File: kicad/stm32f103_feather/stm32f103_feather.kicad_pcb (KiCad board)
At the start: 2 copper layers, 50.8 x 22.9 mm, 34 parts, among them J1 Bottom-conn, J2 Top-conn, J3 Debug-conn, J4 USB_B_Micro, J5 JST-LiPo-conn, SW1 SW_Push, U1 STM32F103CBTx, U2 AMS1117-3.3, U3 MCP73831-2-OT, Y1 8MHz

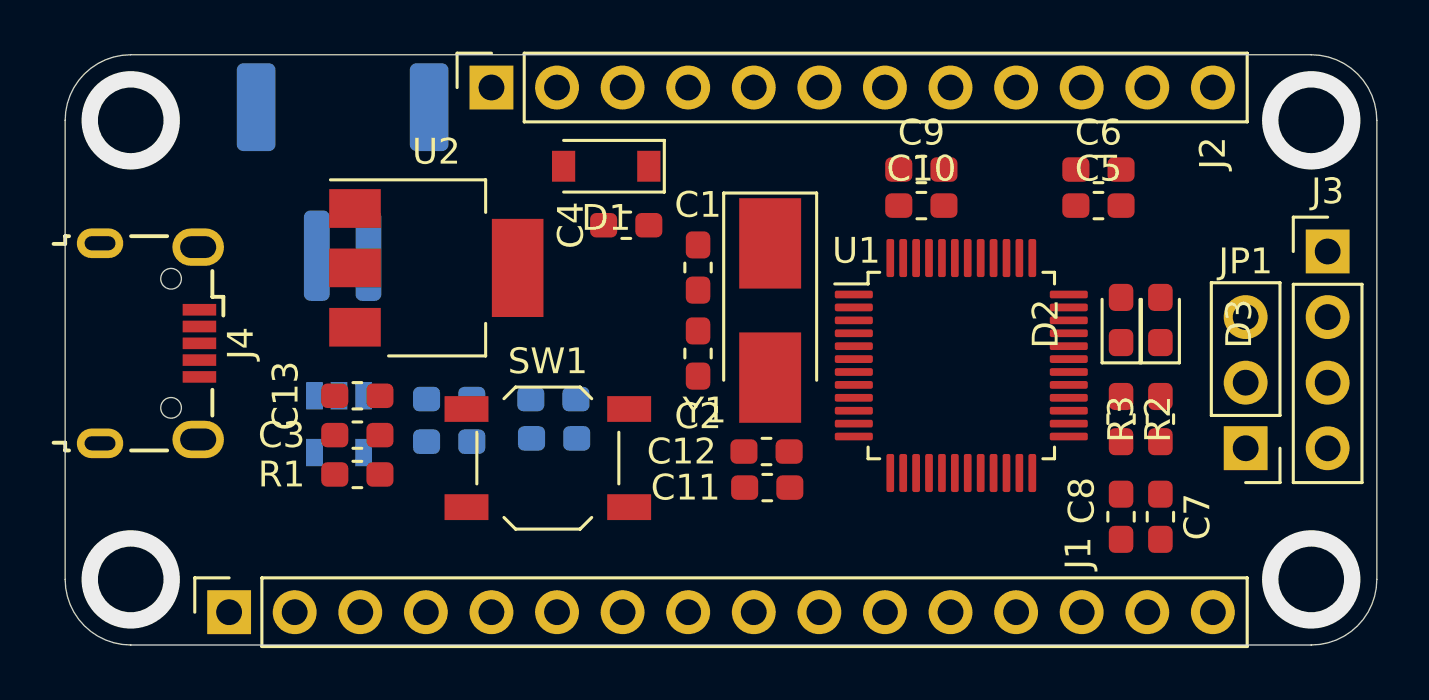
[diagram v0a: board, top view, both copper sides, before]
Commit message: daily update
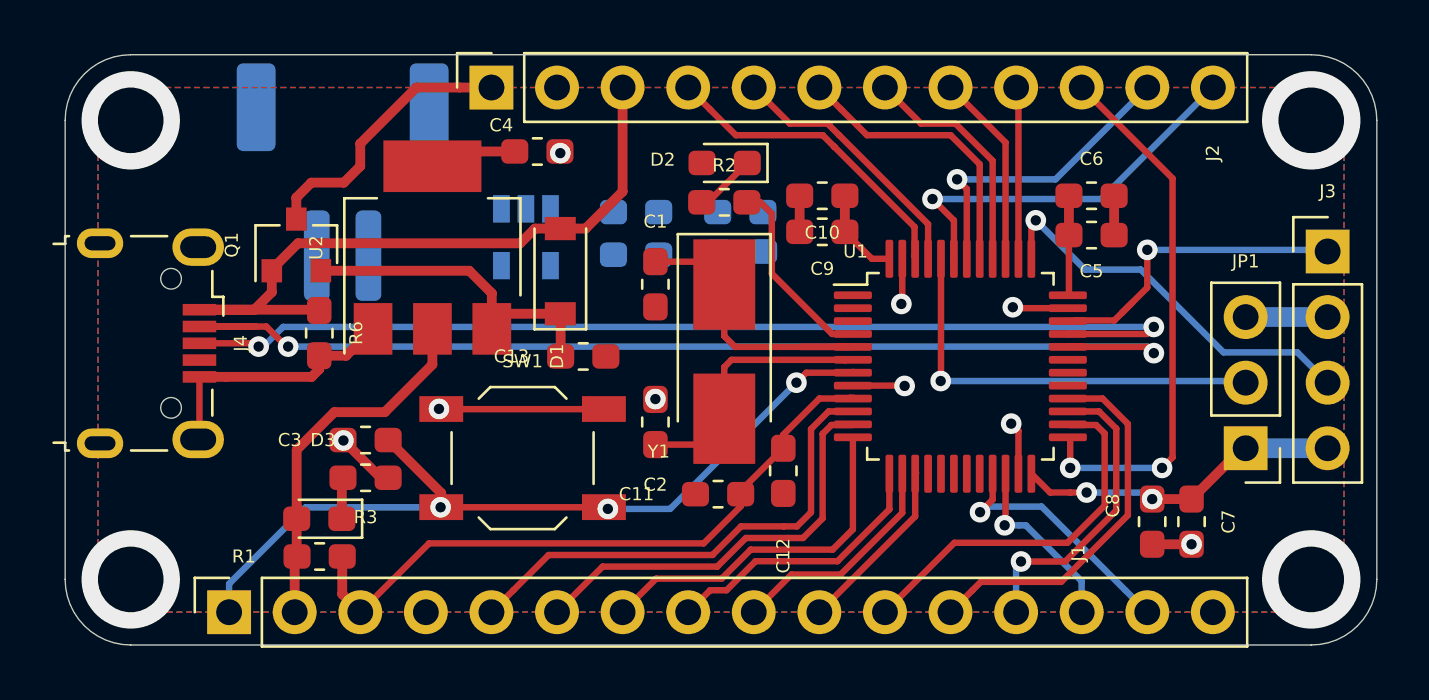
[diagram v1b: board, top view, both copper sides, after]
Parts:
- added Q1: SI2301CDS, Package_TO_SOT_SMD:SOT-23, F.Cu at (136.0, 83.6)
- added R6: 100k, Resistor_SMD:R_0603_1608Metric_Pad1.05x0.95mm_HandSolder, F.Cu at (136.8, 87.0)
- moved D3 33.5 mm to (136.8, 94.2), turned to 180 degrees
- moved R3 30.9 mm to (138.6, 92.6), turned to 0 degrees
- moved R2 17.5 mm to (152.5, 81.9), turned to 0 degrees
- moved D2 16.5 mm to (152.5, 80.4), turned to 180 degrees
- moved R4 10.2 mm to (149.1, 83.9)
- moved C14 10.2 mm to (149.1, 82.3)
- moved R5 10.2 mm to (153.1, 82.3)
- moved U3 10.2 mm to (144.8, 83.3)
- moved D4 10.2 mm to (153.2, 83.8)
- moved C13 8.88 mm to (147.1, 87.9)
- moved C9 4.53 mm to (156.3, 83.1), turned to 180 degrees
- moved C4 4.47 mm to (145.3, 79.9)
- moved D1 4.44 mm to (146.2, 84.6), turned to 90 degrees
- moved C10 3.86 mm to (156.3, 81.7), turned to 180 degrees
- moved R1 3.49 mm to (136.9, 95.6)
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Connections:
- C13 pad 2: /usb -> Net-(C13-Pad2)
- D1 pad 1: /usb -> Net-(C13-Pad2)
- D1 pad 2: /bat -> /usb
- J1 pad 1: (no net) -> /nrst
- J1 pad 4: /gnd -> GND
- J2 pad 4: /pb8 -> /cantx
- J2 pad 5: /pb9 -> /canrx
- J2 pad 6: /pb10 -> /pb5
- J2 pad 7: /pb11 -> /pb4
- J2 pad 8: /pa6 -> /pb3
- J2 pad 9: /pa7 -> /pa15
- J3 pad 2: /gnd -> GND
- R2 pad 2: /pa8 -> /LED
- U1 pad 16: /pa6 -> (no net)
- U1 pad 17: /pa7 -> (no net)
- U1 pad 21: /pb10 -> /tx
- U1 pad 22: /pb11 -> /rx
- U1 pad 29: /pa8 -> (no net)
- U1 pad 3: /osc_in -> (no net)
- U1 pad 30: /tx -> (no net)
- U1 pad 31: /rx -> (no net)
- U1 pad 38: (no net) -> /pa15
- U1 pad 39: (no net) -> /pb3
- U1 pad 4: /osc_out -> /LED
- U1 pad 40: (no net) -> /pb4
- U1 pad 41: (no net) -> /pb5
- U1 pad 45: /pb8 -> /canrx
- U1 pad 46: /pb9 -> /cantx
- U1 pad 5: (no net) -> /osc_in
- U1 pad 6: (no net) -> /osc_out
- U2 pad 3: /usb -> Net-(C13-Pad2)
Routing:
- net /usb_dm: track 0.00 -> 43.1 mm, vias 0 -> 2
- net /usb_dp: track 0.00 -> 40.9 mm, vias 0 -> 2
- net /3vo: track 0.00 -> 38.9 mm, vias 0 -> 2
- net GND: track 0.00 -> 34.6 mm, vias 0 -> 13
- net /nrst: track 0.00 -> 32.1 mm, vias 0 -> 3
- net /usb: track 0.00 -> 27.5 mm
- net /vref: track 0.00 -> 25.8 mm
- net /nss: track 0.00 -> 21.1 mm, vias 0 -> 2
- net /a0: track 0.00 -> 19.1 mm
- net /boot: track 0.00 -> 16.6 mm, vias 0 -> 1
- net /a1: track 0.00 -> 16.4 mm
- net /swclk: track 0.00 -> 15.5 mm, vias 0 -> 1
- net /sda: track 0.00 -> 15.3 mm, vias 0 -> 1
- net /mo: track 0.00 -> 14.7 mm
- net /sck: track 0.00 -> 14.6 mm
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- added copper zone on B.Cu, net GND
- added copper zone on F.Cu, net GND
